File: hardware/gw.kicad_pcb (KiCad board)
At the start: 4 copper layers, 47 x 32.9 mm, 21 parts, among them J1 USB_OTG, J2 Conn_01x04, U1 ESP-12F, U2 Ai-Thinker-Ra-02, U3 AMS1117-3.3

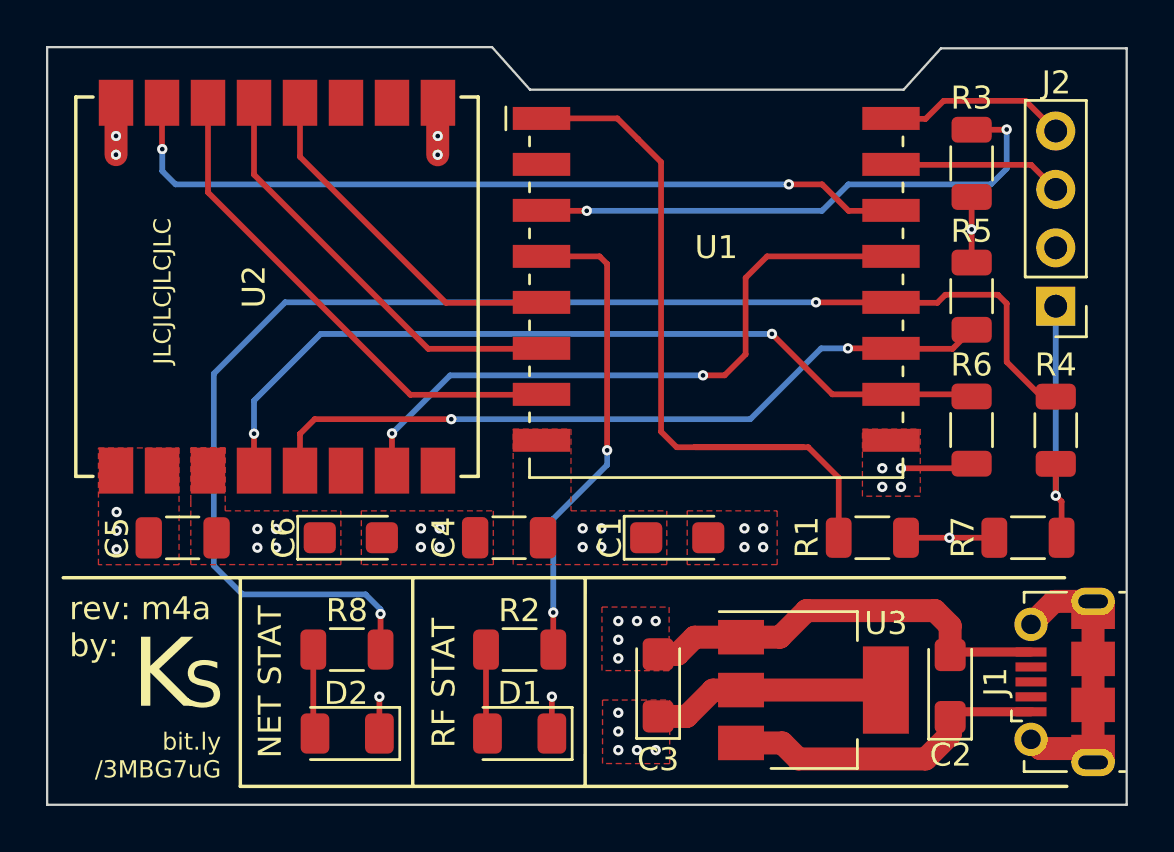
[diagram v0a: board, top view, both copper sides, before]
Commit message: Fixup pins
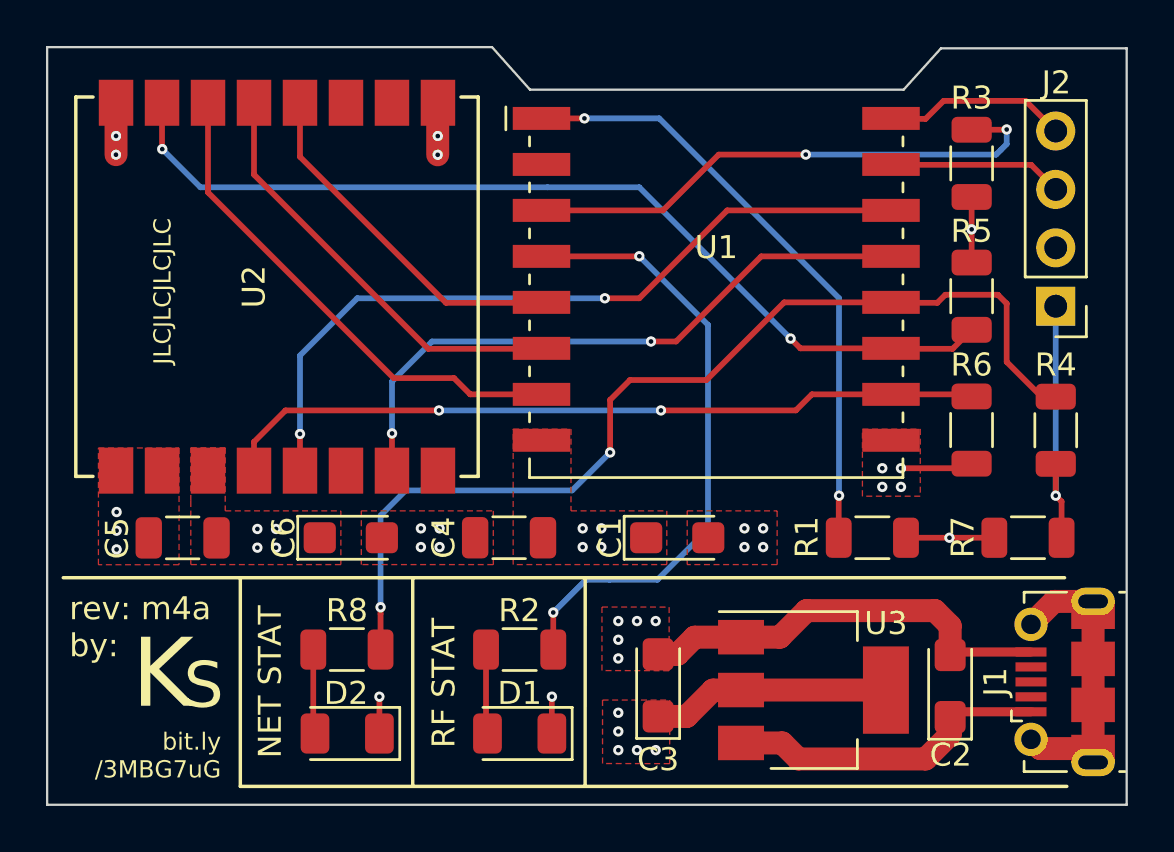
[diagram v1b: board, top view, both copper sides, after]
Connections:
- R5 pad 1: /DIO0 -> /SS
- U1 pad 11: /DIO0 -> /SS
- U1 pad 14: /SS -> /DIO0
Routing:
- net /WF_LED: track 59.5 -> 43.8 mm
- net Net-(R1-Pad2): track 33.6 -> 26.6 mm, vias 0 -> 2
- net /RF_LED: track 20.7 -> 27.2 mm
- net /SS: track 35.4 -> 41.1 mm
- net /RESET: track 36.6 -> 33.4 mm
- net /DIO0: track 32.7 -> 33.3 mm
- net Net-(R3-Pad2): track 24.2 -> 23.6 mm
- net /DIO2: track 28.5 -> 27.8 mm
